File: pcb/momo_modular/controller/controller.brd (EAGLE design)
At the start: 19 parts, among them U6 PIC24F16KA101-X_PSSOP, U7 FLASH8MSOP8

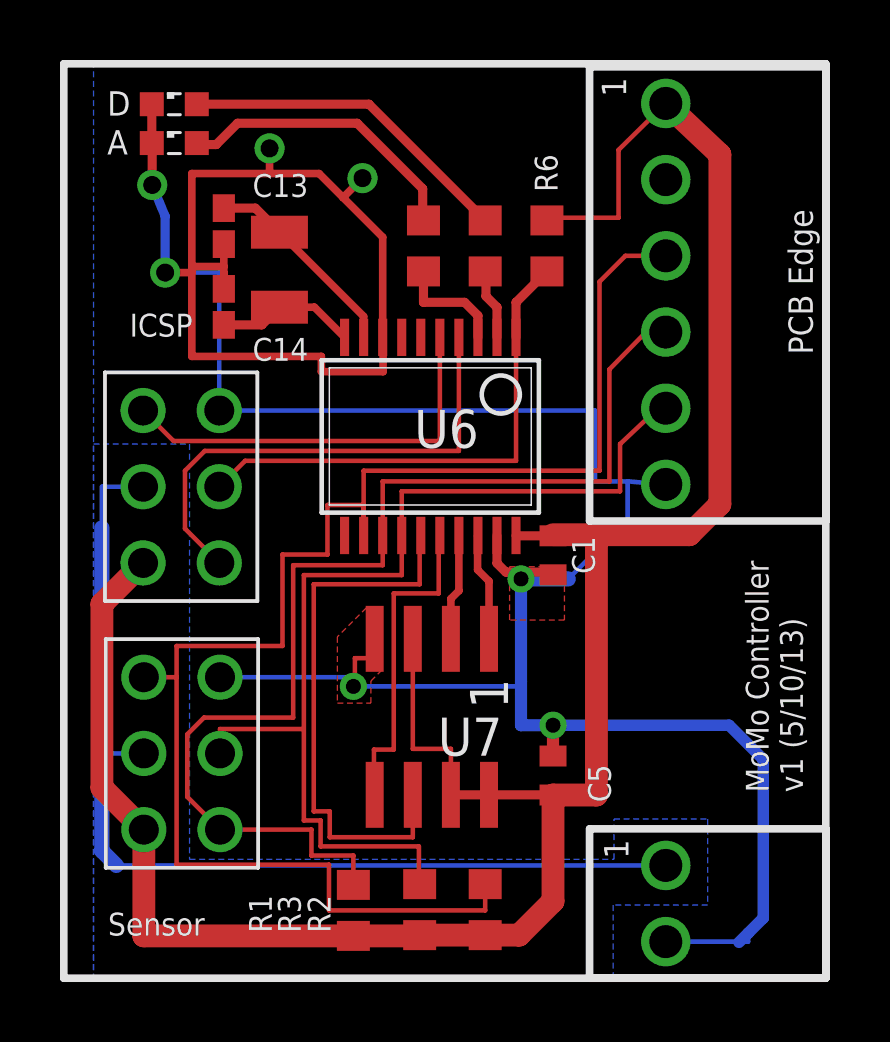
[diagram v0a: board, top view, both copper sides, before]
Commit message: Controller Board v2.1 Done
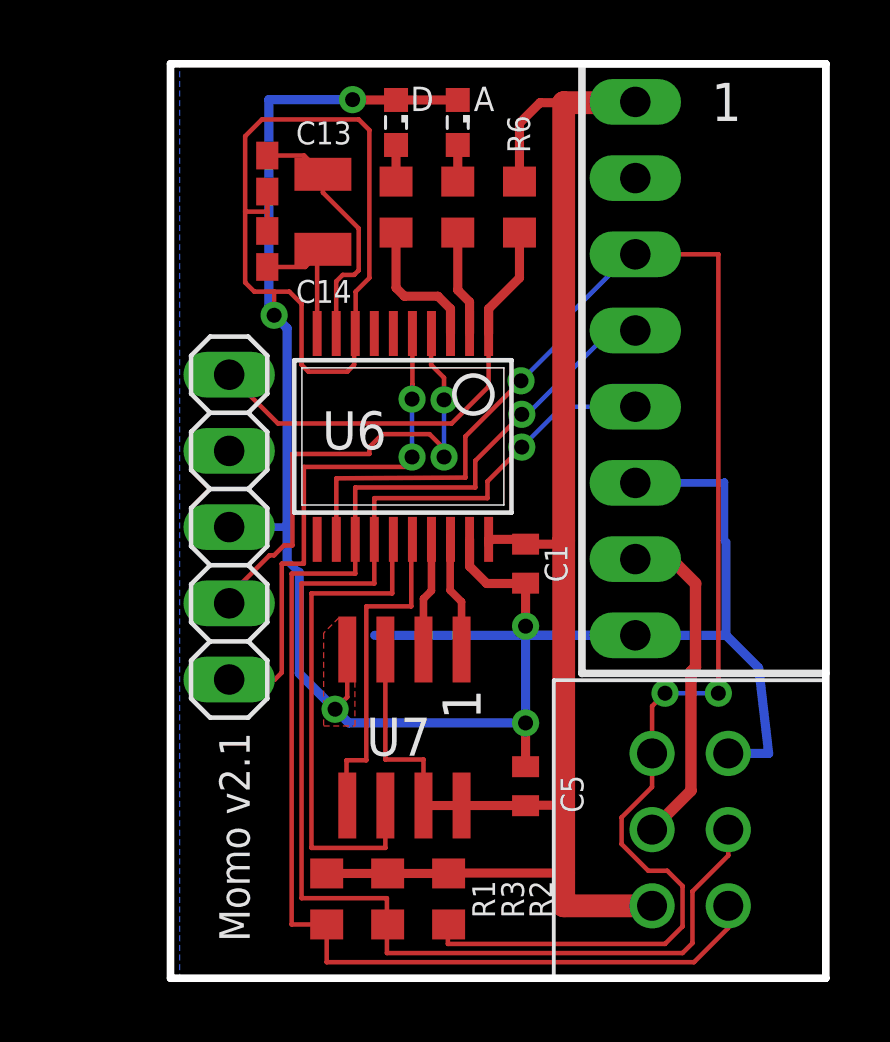
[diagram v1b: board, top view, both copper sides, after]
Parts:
- removed U$2: 2X3-MOLEX-90130, components:2X3-MOLEX-90130
- removed U$4: MOMO-EDGE-SMALL-F, components:MOMO-EDGE-SMALL-6F
- added JP1: (no value), pinhead:1X05
- U$1: value MOMO-EDGE-POWER-F -> MOMO-EDGE-8F; device components:MOMO-EDGE-SMALL-2F -> components:MOMO-EDGE-8F
- moved U$3 17.1 mm to (52.6, 17.1)
- moved U$1 16.6 mm to (49.5, 31.2), turned to 0 degrees
- moved LED2 9.47 mm to (43.6, 40.7), turned to 270 degrees
- moved LED1 7.42 mm to (41.5, 40.7), turned to 270 degrees
- moved C14 2.41 mm to (37.2, 36.5)
- moved XTAL1 2.41 mm to (39.1, 39.0)
- moved C13 2.27 mm to (37.2, 39.0)
- moved R4 1.59 mm to (41.5, 37.9)
- moved R5 1.59 mm to (43.6, 37.9)
- moved R6 1.59 mm to (45.6, 37.9)
- moved R2 1.27 mm to (43.3, 14.8), turned to 90 degrees
- moved R3 1.12 mm to (41.2, 14.8), turned to 90 degrees
- moved C5 0.98 mm to (45.8, 18.6)
- moved U7 0.98 mm to (41.8, 20.5)
- moved R1 0.97 mm to (39.2, 14.8), turned to 90 degrees
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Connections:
- removed net N$18: U$2.3, U6.5
- removed net N$19: U$2.4, U6.4
- removed net NC: U$4.2
- new net N$6: JP1.4, U6.4
- new net N$7: JP1.5, U6.5
- net GND: now also JP1.3, U$1.GND, U$1.PGND; no longer U$1.2, U$2.6, U$4.6
- net ICLK: now also U$1.CLK; no longer U$4.3
- net IDAT: now also U$1.DAT; no longer U$4.4
- net IRQ: now also U$1.ARLM; no longer U$4.5
- net N$15: now also JP1.1; no longer U$2.5
- net V+: now also U$1.V4.; no longer U$1.1, U$2.2
- net VCCINT: now also U$1.V28; no longer U$2.1, U$4.1
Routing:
- net V+: track 33.9 -> 11.1 mm
- net VCCINT: track 79.5 -> 57.8 mm
- net N$7: track 0.00 -> 17.5 mm, vias 0 -> 2
- net N$19: track 16.8 -> 0.00 mm
- net N$6: track 0.00 -> 16.3 mm, vias 0 -> 2
- net N$18: track 13.8 -> 0.00 mm
- net IRQ: track 34.7 -> 45.4 mm, vias 0 -> 1
- net N$1: track 11.2 -> 1.22 mm
- net N$2: track 9.82 -> 1.22 mm
- net IDAT: track 38.2 -> 45.7 mm, vias 0 -> 1
- net GND: track 105.6 -> 103.1 mm, vias 7 -> 5
- net ICLK: track 51.9 -> 53.7 mm, vias 0 -> 3
- net N$15: track 17.0 -> 15.4 mm
- net N$25: track 6.85 -> 8.45 mm
- net SCLK: track 18.3 -> 17.1 mm
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- removed copper zone on layer 16, net V+
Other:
- board outline added: 21.8 x 30.5 mm
- board text added: "Momo v2.1"
- board text removed: "ICSP"
- board text removed: "MoMo Controller v1 (5/10/13)"
- board text removed: "Sensor"

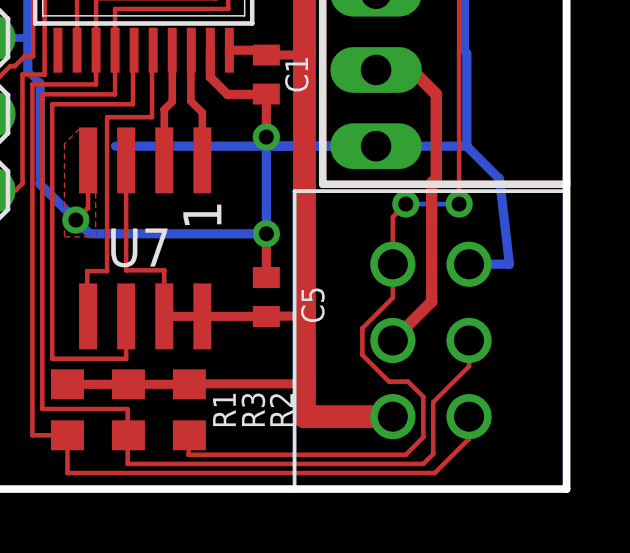
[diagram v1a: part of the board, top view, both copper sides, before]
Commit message: Improved one trace to avoid 2 vias
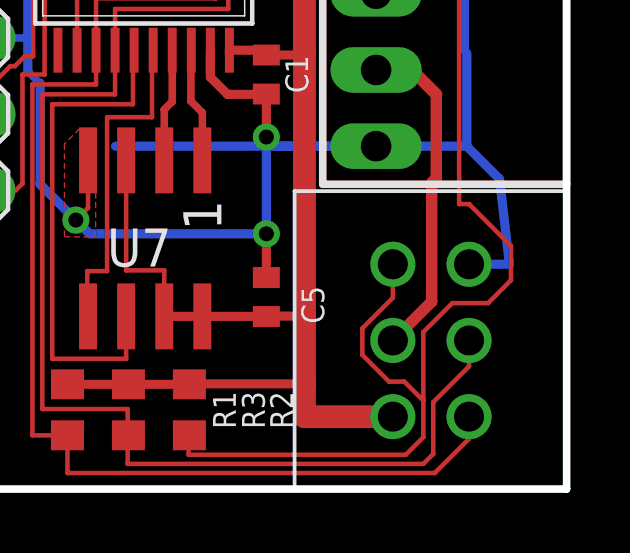
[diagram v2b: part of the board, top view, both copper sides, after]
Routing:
- net ICLK: track 53.7 -> 59.0 mm, vias 3 -> 1
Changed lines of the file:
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@@
 <wire x1="33.9852" y1="42.6466" x2="33.9852" y2="12.1666" width="0.254" layer="20"/>
 <wire x1="33.9852" y1="12.1666" x2="55.8292" y2="12.1666" width="0.254" layer="20"/>
-<dimension x1="34.2392" y1="42.6466" x2="55.88" y2="42.6974" x3="45.0596" y3="44.3992" textsize="1.778" layer="48" dtype="horizontal" unit="inch" precision="3" visible="yes"/>
-<dimension x1="34.2392" y1="12.1666" x2="34.29" y2="42.672" x3="32.5882" y3="27.4193" textsize="1.778" layer="48" dtype="vertical" unit="inch" precision="3" visible="yes"/>
 <text x="36.6268" y="13.3858" size="1.016" layer="21" rot="R90">Momo v2.1</text>
+<dimension x1="33.9852" y1="42.6466" x2="55.8292" y2="42.6466" x3="44.9072" y3="44.6532" textsize="1.6764" layer="49" dtype="horizontal" unit="inch" precision="3" visible="yes"/>
+<dimension x1="33.9852" y1="42.6466" x2="33.9852" y2="12.1666" x3="32.258" y3="27.4066" textsize="1.6764" layer="49" dtype="vertical" unit="inch" precision="3" visible="yes"/>
 </plain>
 <attributes>
@@
 <wire x1="43.2562" y1="13.9582" x2="43.2308" y2="13.9328" width="0.1524" layer="1"/>
 <wire x1="43.2308" y1="13.9328" x2="43.2308" y2="13.3096" width="0.1524" layer="1"/>
-<via x="52.2478" y="21.6662" extent="1-16" drill="0.5"/>
-<wire x1="52.2478" y1="21.6662" x2="50.4698" y2="21.6662" width="0.1524" layer="16"/>
 <wire x1="49.4792" y1="36.2966" x2="49.3014" y2="36.2966" width="0.1524" layer="16"/>
 <wire x1="49.3014" y1="36.2966" x2="47.1932" y2="34.1884" width="0.1524" layer="16"/>
@@
 <wire x1="43.2308" y1="13.3096" x2="50.4698" y2="13.3096" width="0.1524" layer="1"/>
 <wire x1="50.4698" y1="13.3096" x2="51.054" y2="13.8938" width="0.1524" layer="1"/>
-<wire x1="51.054" y1="13.8938" x2="51.054" y2="15.24" width="0.1524" layer="1"/>
-<wire x1="51.054" y1="15.24" x2="50.546" y2="15.748" width="0.1524" layer="1"/>
-<wire x1="50.546" y1="15.748" x2="49.911" y2="15.748" width="0.1524" layer="1"/>
 <wire x1="49.911" y1="15.748" x2="49.022" y2="16.637" width="0.1524" layer="1"/>
 <wire x1="49.022" y1="16.637" x2="49.022" y2="17.526" width="0.1524" layer="1"/>
 <wire x1="49.022" y1="17.526" x2="50.038" y2="18.542" width="0.1524" layer="1"/>
 <wire x1="50.038" y1="18.542" x2="50.038" y2="19.6596" width="0.1524" layer="1"/>
-<via x="50.4698" y="21.6662" extent="1-16" drill="0.5"/>
-<wire x1="50.4698" y1="21.6662" x2="50.038" y2="21.2344" width="0.1524" layer="1"/>
-<wire x1="50.038" y1="21.2344" x2="50.038" y2="19.6596" width="0.1524" layer="1"/>
 <wire x1="49.4792" y1="36.2966" x2="52.2478" y2="36.2966" width="0.1524" layer="1"/>
 <wire x1="52.2478" y1="36.2966" x2="52.2478" y2="21.6662" width="0.1524" layer="1"/>
+<wire x1="52.2478" y1="21.6662" x2="52.578" y2="21.6662" width="0.1524" layer="1"/>
+<wire x1="52.578" y1="21.6662" x2="53.975" y2="20.2692" width="0.1524" layer="1"/>
+<wire x1="53.975" y1="20.2692" x2="53.975" y2="19.1262" width="0.1524" layer="1"/>
+<wire x1="53.975" y1="19.1262" x2="53.213" y2="18.3642" width="0.1524" layer="1"/>
+<wire x1="51.054" y1="17.399" x2="51.054" y2="15.113" width="0.1524" layer="1"/>
+<wire x1="51.054" y1="15.113" x2="51.054" y2="13.8938" width="0.1524" layer="1"/>
+<wire x1="53.213" y1="18.3642" x2="52.0192" y2="18.3642" width="0.1524" layer="1"/>
+<wire x1="52.0192" y1="18.3642" x2="51.054" y2="17.399" width="0.1524" layer="1"/>
+<wire x1="49.911" y1="15.748" x2="50.419" y2="15.748" width="0.1524" layer="1"/>
+<wire x1="50.419" y1="15.748" x2="51.054" y2="15.113" width="0.1524" layer="1"/>
 </signal>
 <signal name="N$4">

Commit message: Revert "Improved one trace to avoid 2 vias"
This reverts commit defd9550a6ffd5e7c1ff802918ca0e38fc084f46.
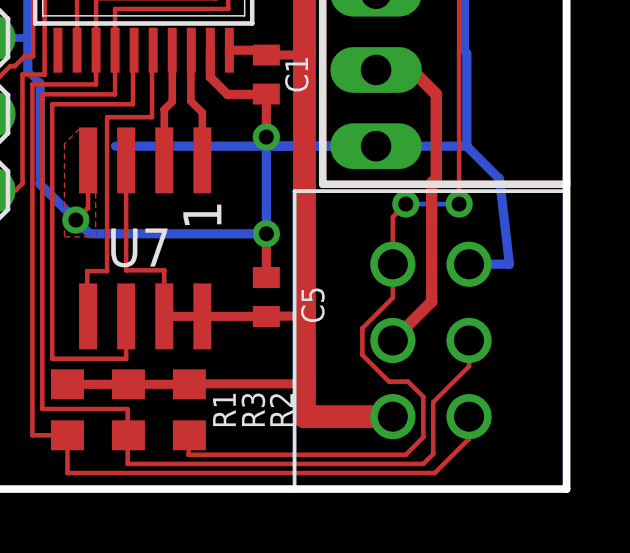
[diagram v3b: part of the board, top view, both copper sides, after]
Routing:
- net ICLK: track 59.0 -> 53.7 mm, vias 1 -> 3
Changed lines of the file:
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@@
 <wire x1="33.9852" y1="42.6466" x2="33.9852" y2="12.1666" width="0.254" layer="20"/>
 <wire x1="33.9852" y1="12.1666" x2="55.8292" y2="12.1666" width="0.254" layer="20"/>
+<dimension x1="34.2392" y1="42.6466" x2="55.88" y2="42.6974" x3="45.0596" y3="44.3992" textsize="1.778" layer="48" dtype="horizontal" unit="inch" precision="3" visible="yes"/>
+<dimension x1="34.2392" y1="12.1666" x2="34.29" y2="42.672" x3="32.5882" y3="27.4193" textsize="1.778" layer="48" dtype="vertical" unit="inch" precision="3" visible="yes"/>
 <text x="36.6268" y="13.3858" size="1.016" layer="21" rot="R90">Momo v2.1</text>
-<dimension x1="33.9852" y1="42.6466" x2="55.8292" y2="42.6466" x3="44.9072" y3="44.6532" textsize="1.6764" layer="49" dtype="horizontal" unit="inch" precision="3" visible="yes"/>
-<dimension x1="33.9852" y1="42.6466" x2="33.9852" y2="12.1666" x3="32.258" y3="27.4066" textsize="1.6764" layer="49" dtype="vertical" unit="inch" precision="3" visible="yes"/>
 </plain>
 <attributes>
@@
 <wire x1="43.2562" y1="13.9582" x2="43.2308" y2="13.9328" width="0.1524" layer="1"/>
 <wire x1="43.2308" y1="13.9328" x2="43.2308" y2="13.3096" width="0.1524" layer="1"/>
+<via x="52.2478" y="21.6662" extent="1-16" drill="0.5"/>
+<wire x1="52.2478" y1="21.6662" x2="50.4698" y2="21.6662" width="0.1524" layer="16"/>
 <wire x1="49.4792" y1="36.2966" x2="49.3014" y2="36.2966" width="0.1524" layer="16"/>
 <wire x1="49.3014" y1="36.2966" x2="47.1932" y2="34.1884" width="0.1524" layer="16"/>
@@
 <wire x1="43.2308" y1="13.3096" x2="50.4698" y2="13.3096" width="0.1524" layer="1"/>
 <wire x1="50.4698" y1="13.3096" x2="51.054" y2="13.8938" width="0.1524" layer="1"/>
+<wire x1="51.054" y1="13.8938" x2="51.054" y2="15.24" width="0.1524" layer="1"/>
+<wire x1="51.054" y1="15.24" x2="50.546" y2="15.748" width="0.1524" layer="1"/>
+<wire x1="50.546" y1="15.748" x2="49.911" y2="15.748" width="0.1524" layer="1"/>
 <wire x1="49.911" y1="15.748" x2="49.022" y2="16.637" width="0.1524" layer="1"/>
 <wire x1="49.022" y1="16.637" x2="49.022" y2="17.526" width="0.1524" layer="1"/>
 <wire x1="49.022" y1="17.526" x2="50.038" y2="18.542" width="0.1524" layer="1"/>
 <wire x1="50.038" y1="18.542" x2="50.038" y2="19.6596" width="0.1524" layer="1"/>
+<via x="50.4698" y="21.6662" extent="1-16" drill="0.5"/>
+<wire x1="50.4698" y1="21.6662" x2="50.038" y2="21.2344" width="0.1524" layer="1"/>
+<wire x1="50.038" y1="21.2344" x2="50.038" y2="19.6596" width="0.1524" layer="1"/>
 <wire x1="49.4792" y1="36.2966" x2="52.2478" y2="36.2966" width="0.1524" layer="1"/>
 <wire x1="52.2478" y1="36.2966" x2="52.2478" y2="21.6662" width="0.1524" layer="1"/>
-<wire x1="52.2478" y1="21.6662" x2="52.578" y2="21.6662" width="0.1524" layer="1"/>
-<wire x1="52.578" y1="21.6662" x2="53.975" y2="20.2692" width="0.1524" layer="1"/>
-<wire x1="53.975" y1="20.2692" x2="53.975" y2="19.1262" width="0.1524" layer="1"/>
-<wire x1="53.975" y1="19.1262" x2="53.213" y2="18.3642" width="0.1524" layer="1"/>
-<wire x1="51.054" y1="17.399" x2="51.054" y2="15.113" width="0.1524" layer="1"/>
-<wire x1="51.054" y1="15.113" x2="51.054" y2="13.8938" width="0.1524" layer="1"/>
-<wire x1="53.213" y1="18.3642" x2="52.0192" y2="18.3642" width="0.1524" layer="1"/>
-<wire x1="52.0192" y1="18.3642" x2="51.054" y2="17.399" width="0.1524" layer="1"/>
-<wire x1="49.911" y1="15.748" x2="50.419" y2="15.748" width="0.1524" layer="1"/>
-<wire x1="50.419" y1="15.748" x2="51.054" y2="15.113" width="0.1524" layer="1"/>
 </signal>
 <signal name="N$4">
